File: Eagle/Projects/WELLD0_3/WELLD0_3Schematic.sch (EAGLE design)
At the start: 31 parts, among them IC1 STM32F030F4P6TR, U2 CJT1117-3.3-SOT223

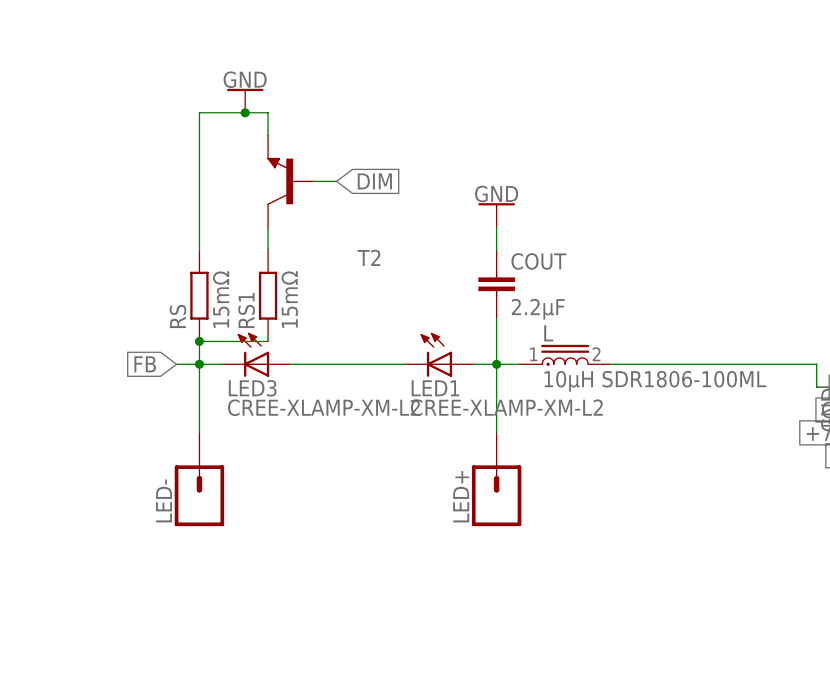
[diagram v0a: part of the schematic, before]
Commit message: Ordered PCB
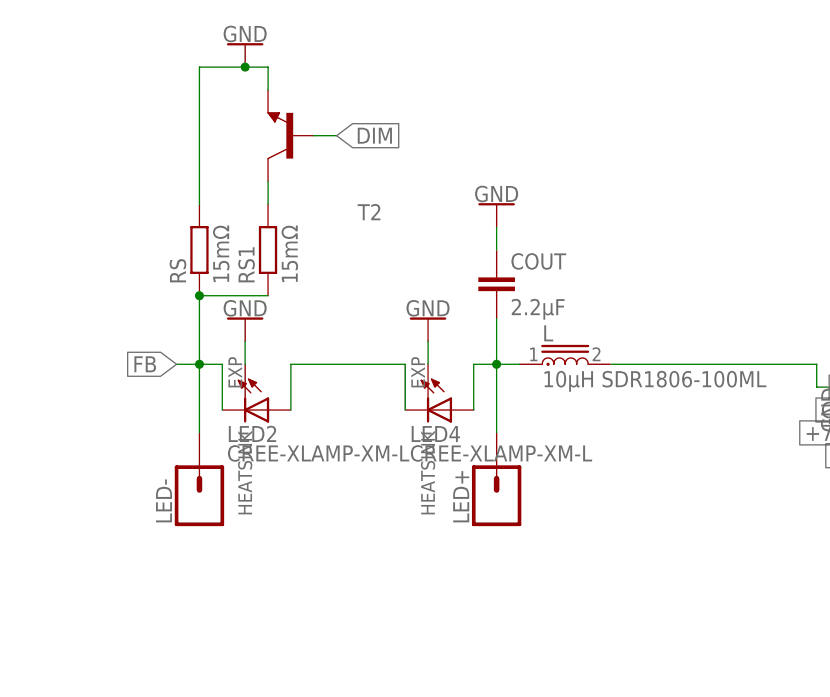
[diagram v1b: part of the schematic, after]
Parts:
- removed LED1, LED3: CREE-XLAMP-XM-L2, led:CREE-XLAMP-XM-L
- added LED2, LED4: CREE-XLAMP-XM-L, led1:CREE-XLAMP-XM-L
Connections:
- net FB: now also LED2.C; no longer LED3.C
- net GND: now also LED2.HEATSINK, LED4.HEATSINK
- net N$1: now also LED4.A; no longer LED1.A
- net N$2: now also LED2.A, LED4.C; no longer LED1.C, LED3.A
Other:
- moved on the sheet: RS, RS1, T2
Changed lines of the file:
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@@
 <part name="ST1CC40" library="SparkFun-Retired" deviceset="GENERIC-SOIC8" device="MSGEQ7N-FILTER"/>
 <part name="GND1" library="SparkFun-PowerSymbols" library_urn="urn:adsk.eagle:library:530" deviceset="GND" device=""/>
-<part name="LED1" library="led" library_urn="urn:adsk.eagle:library:259" deviceset="CREE-XLAMP-XM-L" device="" package3d_urn="urn:adsk.eagle:package:15887/1" value="CREE-XLAMP-XM-L2"/>
-<part name="LED3" library="led" library_urn="urn:adsk.eagle:library:259" deviceset="CREE-XLAMP-XM-L" device="" package3d_urn="urn:adsk.eagle:package:15887/1" value="CREE-XLAMP-XM-L2"/>
 <part name="L" library="SDR1806-470ML" deviceset="SDR1806-470ML" device="" value="10µH SDR1806-100ML"/>
 <part name="COUT" library="rcl" library_urn="urn:adsk.eagle:library:334" deviceset="C-EU" device="C0603" package3d_urn="urn:adsk.eagle:package:23616/2" value="2.2µF"/>
@@
 <part name="GND7" library="SparkFun-PowerSymbols" library_urn="urn:adsk.eagle:library:530" deviceset="GND" device=""/>
 <part name="SV1" library="con-lstb" library_urn="urn:adsk.eagle:library:162" deviceset="MA06-1" device="" package3d_urn="urn:adsk.eagle:package:8340/1"/>
+<part name="LED2" library="led1" deviceset="CREE-XLAMP-XM-L" device="" package3d_urn="urn:adsk.eagle:package:15887/1"/>
+<part name="LED4" library="led1" deviceset="CREE-XLAMP-XM-L" device="" package3d_urn="urn:adsk.eagle:package:15887/1"/>
+<part name="GND11" library="SparkFun-PowerSymbols" library_urn="urn:adsk.eagle:library:530" deviceset="GND" device=""/>
+<part name="GND13" library="SparkFun-PowerSymbols" library_urn="urn:adsk.eagle:library:530" deviceset="GND" device=""/>
 </parts>
 <sheets>
@@
 <attribute name="VALUE" x="150.114" y="81.28" size="1.778" layer="96" rot="R90" align="top-center"/>
 </instance>
-<instance part="LED1" gate="G$1" x="73.66" y="86.36" rot="R270">
-<attribute name="NAME" x="69.088" y="82.804" size="1.778" layer="95"/>
-<attribute name="VALUE" x="69.088" y="80.645" size="1.778" layer="96"/>
-</instance>
-<instance part="LED3" gate="G$1" x="53.34" y="86.36" rot="R270">
-<attribute name="NAME" x="48.768" y="82.804" size="1.778" layer="95"/>
-<attribute name="VALUE" x="48.768" y="80.645" size="1.778" layer="96"/>
-</instance>
 <instance part="L" gate="G$1" x="86.36" y="86.36">
 <attribute name="NAME" x="83.812790625" y="88.907209375" size="1.78305" layer="95"/>
@@
 <attribute name="VALUE" x="80.264" y="91.821" size="1.778" layer="96"/>
 </instance>
-<instance part="RS" gate="G$1" x="45.72" y="93.98" rot="R90">
-<attribute name="NAME" x="44.2214" y="90.17" size="1.778" layer="95" rot="R90"/>
-<attribute name="VALUE" x="49.022" y="90.17" size="1.778" layer="96" rot="R90"/>
-</instance>
-<instance part="GND2" gate="1" x="50.8" y="116.84" rot="R180">
-<attribute name="VALUE" x="50.8" y="117.094" size="1.778" layer="96" rot="R180" align="top-center"/>
+<instance part="RS" gate="G$1" x="45.72" y="99.06" rot="R90">
+<attribute name="NAME" x="44.2214" y="95.25" size="1.778" layer="95" rot="R90"/>
+<attribute name="VALUE" x="49.022" y="95.25" size="1.778" layer="96" rot="R90"/>
+</instance>
+<instance part="GND2" gate="1" x="50.8" y="121.92" rot="R180">
+<attribute name="VALUE" x="50.8" y="122.174" size="1.778" layer="96" rot="R180" align="top-center"/>
 </instance>
 <instance part="GND3" gate="1" x="78.74" y="104.14" rot="R180">
@@
 <attribute name="VALUE" x="81.28" y="39.37" size="1.27" layer="96"/>
 </instance>
-<instance part="T2" gate="G$1" x="55.88" y="106.68" rot="R180">
-<attribute name="NAME" x="66.04" y="99.06" size="1.778" layer="95" rot="R180"/>
-<attribute name="VALUE" x="66.04" y="101.6" size="1.778" layer="96" rot="R180"/>
+<instance part="T2" gate="G$1" x="55.88" y="111.76" rot="R180">
+<attribute name="NAME" x="66.04" y="104.14" size="1.778" layer="95" rot="R180"/>
+<attribute name="VALUE" x="66.04" y="106.68" size="1.778" layer="96" rot="R180"/>
 </instance>
 <instance part="BAT+" gate="-1" x="-71.12" y="58.42">
@@
 <attribute name="NAME" x="-68.58" y="52.578" size="1.524" layer="95"/>
 </instance>
-<instance part="RS1" gate="G$1" x="53.34" y="93.98" rot="R90">
-<attribute name="NAME" x="51.8414" y="90.17" size="1.778" layer="95" rot="R90"/>
-<attribute name="VALUE" x="56.642" y="90.17" size="1.778" layer="96" rot="R90"/>
+<instance part="RS1" gate="G$1" x="53.34" y="99.06" rot="R90">
+<attribute name="NAME" x="51.8414" y="95.25" size="1.778" layer="95" rot="R90"/>
+<attribute name="VALUE" x="56.642" y="95.25" size="1.778" layer="96" rot="R90"/>
 </instance>
 <instance part="IC1" gate="G$1" x="-30.48" y="17.78">
@@
 <attribute name="VALUE" x="-102.87" y="-12.7" size="1.778" layer="96"/>
 <attribute name="NAME" x="-102.87" y="8.382" size="1.778" layer="95"/>
+</instance>
+<instance part="LED2" gate="G$1" x="53.34" y="81.28" rot="R270">
+<attribute name="NAME" x="48.768" y="77.724" size="1.778" layer="95"/>
+<attribute name="VALUE" x="48.768" y="75.565" size="1.778" layer="96"/>
+</instance>
+<instance part="LED4" gate="G$1" x="73.66" y="81.28" rot="R270">
+<attribute name="NAME" x="69.088" y="77.724" size="1.778" layer="95"/>
+<attribute name="VALUE" x="69.088" y="75.565" size="1.778" layer="96"/>
+</instance>
+<instance part="GND11" gate="1" x="50.8" y="91.44" rot="R180">
+<attribute name="VALUE" x="50.8" y="91.694" size="1.778" layer="96" rot="R180" align="top-center"/>
+</instance>
+<instance part="GND13" gate="1" x="71.12" y="91.44" rot="R180">
+<attribute name="VALUE" x="71.12" y="91.694" size="1.778" layer="96" rot="R180" align="top-center"/>
 </instance>
 </instances>
@@
 <pinref part="T2" gate="G$1" pin="E"/>
 <pinref part="GND2" gate="1" pin="GND"/>
-<wire x1="53.34" y1="111.76" x2="53.34" y2="114.3" width="0.1524" layer="91"/>
-<wire x1="53.34" y1="114.3" x2="50.8" y2="114.3" width="0.1524" layer="91"/>
+<wire x1="53.34" y1="116.84" x2="53.34" y2="119.38" width="0.1524" layer="91"/>
+<wire x1="53.34" y1="119.38" x2="50.8" y2="119.38" width="0.1524" layer="91"/>
 <pinref part="RS" gate="G$1" pin="2"/>
-<wire x1="45.72" y1="99.06" x2="45.72" y2="114.3" width="0.1524" layer="91"/>
-<wire x1="45.72" y1="114.3" x2="50.8" y2="114.3" width="0.1524" layer="91"/>
-<junction x="50.8" y="114.3"/>
+<wire x1="45.72" y1="104.14" x2="45.72" y2="119.38" width="0.1524" layer="91"/>
+<wire x1="45.72" y1="119.38" x2="50.8" y2="119.38" width="0.1524" layer="91"/>
+<junction x="50.8" y="119.38"/>
 </segment>
 <segment>
@@
 <label x="96.52" y="35.56" size="1.778" layer="95" xref="yes"/>
 </segment>
+<segment>
+<pinref part="GND11" gate="1" pin="GND"/>
+<pinref part="LED2" gate="G$1" pin="HEATSINK"/>
+<wire x1="50.8" y1="88.9" x2="50.8" y2="86.36" width="0.1524" layer="91"/>
+</segment>
+<segment>
+<pinref part="GND13" gate="1" pin="GND"/>
+<pinref part="LED4" gate="G$1" pin="HEATSINK"/>
+<wire x1="71.12" y1="88.9" x2="71.12" y2="86.36" width="0.1524" layer="91"/>
+</segment>
 </net>
 <net name="FB" class="0">
@@
 </segment>
 <segment>
-<pinref part="LED3" gate="G$1" pin="C"/>
 <label x="43.18" y="86.36" size="1.778" layer="95" rot="R180" xref="yes"/>
 <wire x1="48.26" y1="86.36" x2="45.72" y2="86.36" width="0.1524" layer="91"/>
 <pinref part="RS" gate="G$1" pin="1"/>
 <wire x1="45.72" y1="86.36" x2="43.18" y2="86.36" width="0.1524" layer="91"/>
-<wire x1="45.72" y1="88.9" x2="45.72" y2="86.36" width="0.1524" layer="91"/>
+<wire x1="45.72" y1="93.98" x2="45.72" y2="86.36" width="0.1524" layer="91"/>
 <junction x="45.72" y="86.36"/>
 <pinref part="RS1" gate="G$1" pin="1"/>
-<wire x1="53.34" y1="88.9" x2="45.72" y2="88.9" width="0.1524" layer="91"/>
-<junction x="45.72" y="88.9"/>
+<wire x1="53.34" y1="93.98" x2="45.72" y2="93.98" width="0.1524" layer="91"/>
+<junction x="45.72" y="93.98"/>
 <pinref part="LED-" gate="G$1" pin="1"/>
 <wire x1="45.72" y1="86.36" x2="45.72" y2="78.74" width="0.1524" layer="91"/>
+<pinref part="LED2" gate="G$1" pin="C"/>
+<wire x1="48.26" y1="86.36" x2="48.26" y2="81.28" width="0.1524" layer="91"/>
 </segment>
 </net>
@@
 <segment>
 <pinref part="L" gate="G$1" pin="1"/>
-<pinref part="LED1" gate="G$1" pin="A"/>
 <wire x1="81.28" y1="86.36" x2="78.74" y2="86.36" width="0.1524" layer="91"/>
 <pinref part="COUT" gate="G$1" pin="2"/>
@@
 <pinref part="LED+" gate="G$1" pin="1"/>
 <wire x1="78.74" y1="86.36" x2="78.74" y2="78.74" width="0.1524" layer="91"/>
+<pinref part="LED4" gate="G$1" pin="A"/>
+<wire x1="76.2" y1="81.28" x2="76.2" y2="86.36" width="0.1524" layer="91"/>
 </segment>
 </net>
 <net name="N$2" class="0">
 <segment>
-<pinref part="LED1" gate="G$1" pin="C"/>
-<pinref part="LED3" gate="G$1" pin="A"/>
 <wire x1="68.58" y1="86.36" x2="55.88" y2="86.36" width="0.1524" layer="91"/>
+<pinref part="LED2" gate="G$1" pin="A"/>
+<wire x1="55.88" y1="86.36" x2="55.88" y2="81.28" width="0.1524" layer="91"/>
+<pinref part="LED4" gate="G$1" pin="C"/>
+<wire x1="68.58" y1="86.36" x2="68.58" y2="81.28" width="0.1524" layer="91"/>
 </segment>
 </net>
@@
 <pinref part="RS1" gate="G$1" pin="2"/>
 <pinref part="T2" gate="G$1" pin="C"/>
-<wire x1="53.34" y1="99.06" x2="53.34" y2="101.6" width="0.1524" layer="91"/>
+<wire x1="53.34" y1="104.14" x2="53.34" y2="106.68" width="0.1524" layer="91"/>
 </segment>
 </net>
@@
 <segment>
 <pinref part="T2" gate="G$1" pin="B"/>
-<wire x1="58.42" y1="106.68" x2="60.96" y2="106.68" width="0.1524" layer="91"/>
-<label x="60.96" y="106.68" size="1.778" layer="95" xref="yes"/>
-</segment>
-<segment>
+<wire x1="58.42" y1="111.76" x2="60.96" y2="111.76" width="0.1524" layer="91"/>
+<label x="60.96" y="111.76" size="1.778" layer="95" xref="yes"/>
+</segment>
+<segment>
